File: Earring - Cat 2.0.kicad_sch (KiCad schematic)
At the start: 11 parts, among them Q1 2N3904U, Q2 2N3904U

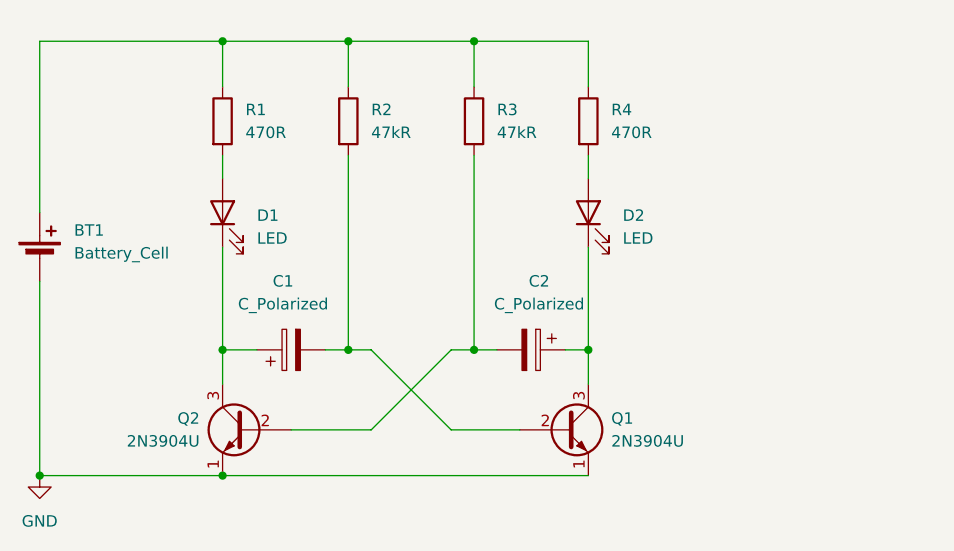
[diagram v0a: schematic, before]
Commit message: render
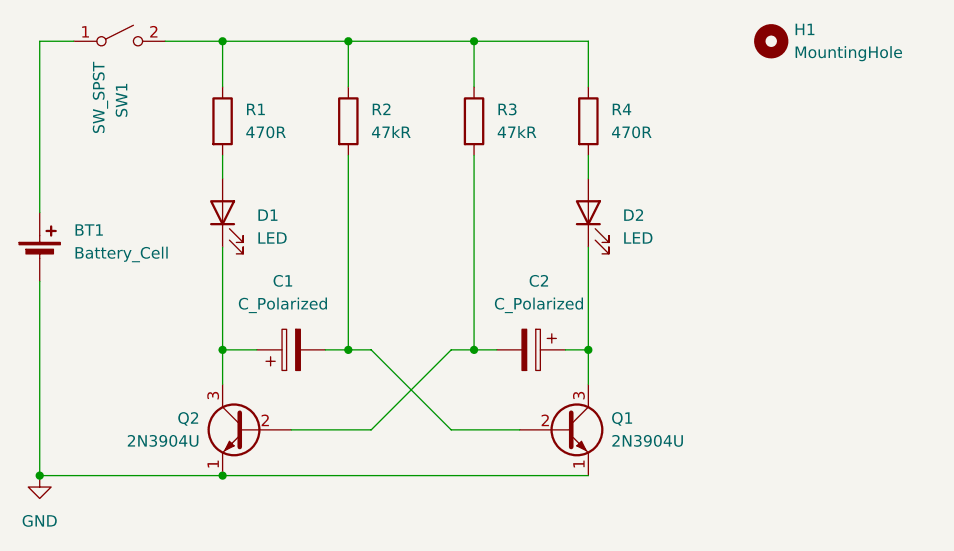
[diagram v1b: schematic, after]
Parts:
- added H1: MountingHole, MountingHole:MountingHole_2.2mm_M2_DIN965_Pad, symbol Mechanical:MountingHole
- added SW1: SW_SPST, Soso:DIP switch 1P THT, symbol Switch:SW_SPST
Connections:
- net at R1.1, R2.1, R3.1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: now also SW1.2 (B); no longer BT1.1 (+)
- new net: BT1.1 (+), SW1.1 (A)
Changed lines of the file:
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@@
 	(wire
 		(pts
-			(xy 71.12 38.1) (xy 91.44 38.1)
+			(xy 71.12 38.1) (xy 74.93 38.1)
 		)
 		(stroke
@@
 		(pts
 			(xy 105.41 50.8) (xy 105.41 72.39)
+		)
+		(stroke
+			(width 0)
+			(type default)
+		)
+	)
+	(wire
+		(pts
+			(xy 85.09 38.1) (xy 91.44 38.1)
 		)
 		(stroke
@@
 					(unit 1)
 				)
+			)
+		)
+	)
+	(symbol
+		(lib_id "Switch:SW_SPST")
+		(at 80.01 38.1 0)
+		(unit 1)
+		(exclude_from_sim no)
+		(in_bom yes)
+		(on_board yes)
+		(dnp no)
+		(property "Reference" "SW1"
+			(at 80.264 42.672 90)
+			(effects
+				(font
+					(size 1.27 1.27)
+				)
+				(justify right)
+			)
+		)
+		(property "Value" "SW_SPST"
+			(at 77.724 40.386 90)
+			(effects
+				(font
+					(size 1.27 1.27)
+				)
+				(justify right)
+			)
+		)
+		(property "Footprint" "Soso:DIP switch 1P THT"
+			(at 80.01 38.1 0)
+			(effects
+				(font
+					(size 1.27 1.27)
+				)
+				(hide yes)
+			)
+		)
+		(property "Datasheet" "~"
+			(at 80.01 38.1 0)
+			(effects
+				(font
+					(size 1.27 1.27)
+				)
+				(hide yes)
+			)
+		)
+		(property "Description" "Single Pole Single Throw (SPST) switch"
+			(at 80.01 38.1 0)
+			(effects
+				(font
+					(size 1.27 1.27)
+				)
+				(hide yes)
+			)
+		)
+		(pin "2"
+		)
+		(pin "1"
+		)
+		(instances
+			(project "Earring - Cat 2.0"
+				(path "/ff3e0cf6-72c2-4d8a-868c-e0988eb4f32e"
+					(reference "SW1")
+					(unit 1)
+				)
+			)
+		)
+	)
+	(symbol
+		(lib_id "Mechanical:MountingHole")
+		(at 152.4 38.1 0)
+		(unit 1)
+		(exclude_from_sim yes)
+		(in_bom no)
+		(on_board yes)
+		(dnp no)
+		(fields_autoplaced yes)
+		(property "Reference" "H1"
+			(at 154.94 36.8299 0)
+			(effects
+				(font
+					(size 1.27 1.27)
+				)
+				(justify left)
+			)
+		)
+		(property "Value" "MountingHole"
+			(at 154.94 39.3699 0)
+			(effects
+				(font
+					(size 1.27 1.27)
+				)
+				(justify left)
+			)
+		)
+		(property "Footprint" "MountingHole:MountingHole_2.2mm_M2_DIN965_Pad"
+			(at 152.4 38.1 0)
+			(effects
+				(font
+					(size 1.27 1.27)
+				)
+				(hide yes)
+			)
+		)
+		(property "Datasheet" "~"
+			(at 152.4 38.1 0)
+			(effects
+				(font
+					(size 1.27 1.27)
+				)
+				(hide yes)
+			)
+		)
+		(property "Description" "Mounting Hole without connection"
+			(at 152.4 38.1 0)
+			(effects
+				(font
+					(size 1.27 1.27)
+				)
+				(hide yes)
+			)
+		)
+		(instances
+			(project ""
+				(path "/ff3e0cf6-72c2-4d8a-868c-e0988eb4f32e"
+					(reference "H1")
+					(unit 1)
+				)
